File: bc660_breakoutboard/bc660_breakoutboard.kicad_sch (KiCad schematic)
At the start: 23 parts, among them J2 Conn_01x12_Pin, J3 Conn_Coaxial, J4 SIM8051-6-0-14-01-X-REVD, U1 BC660K-GL, U2 ESDS304DBVR

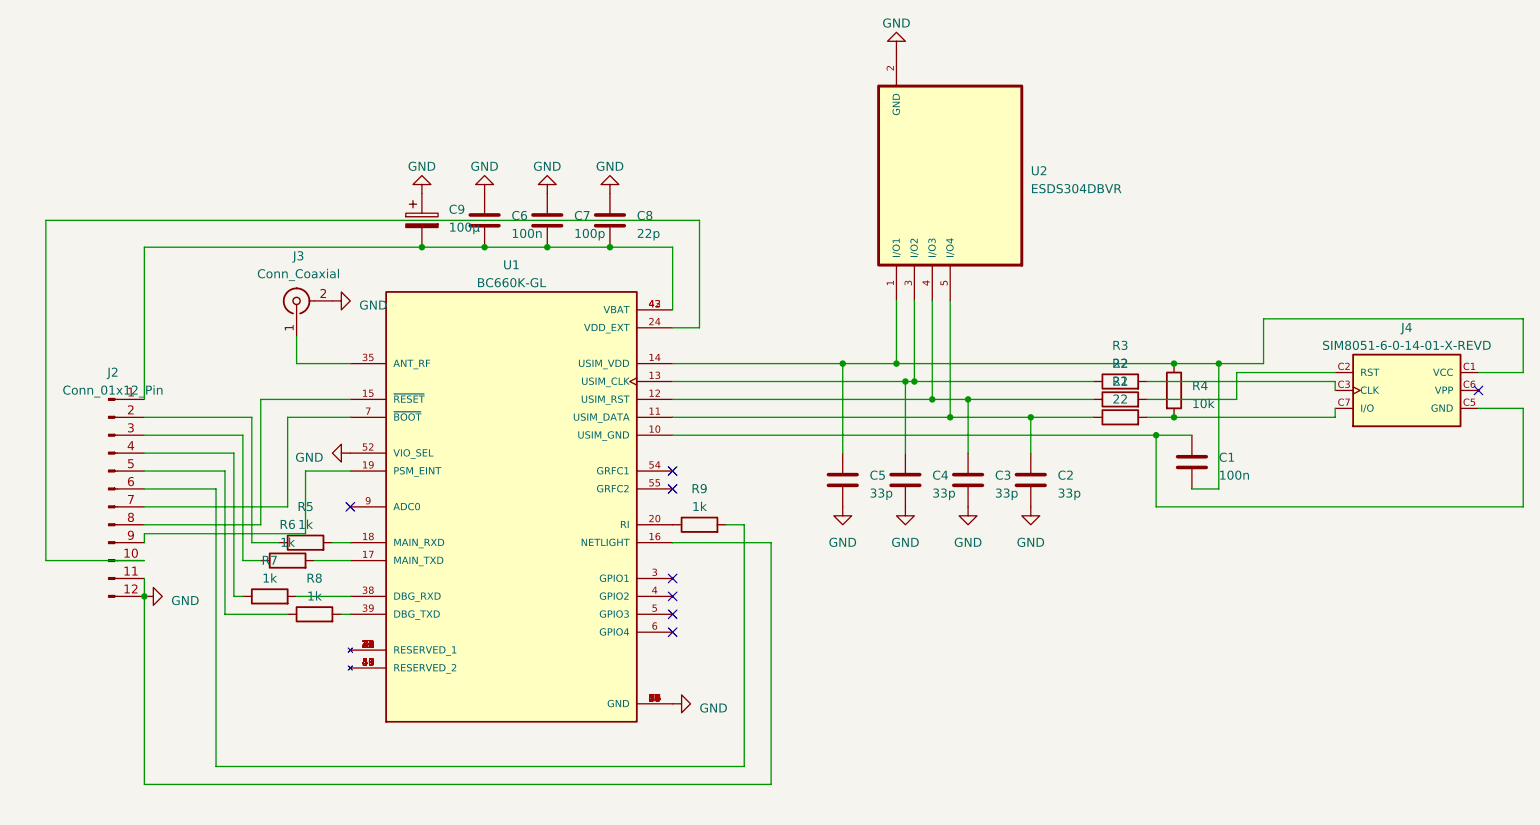
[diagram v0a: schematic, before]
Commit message: update pcb design
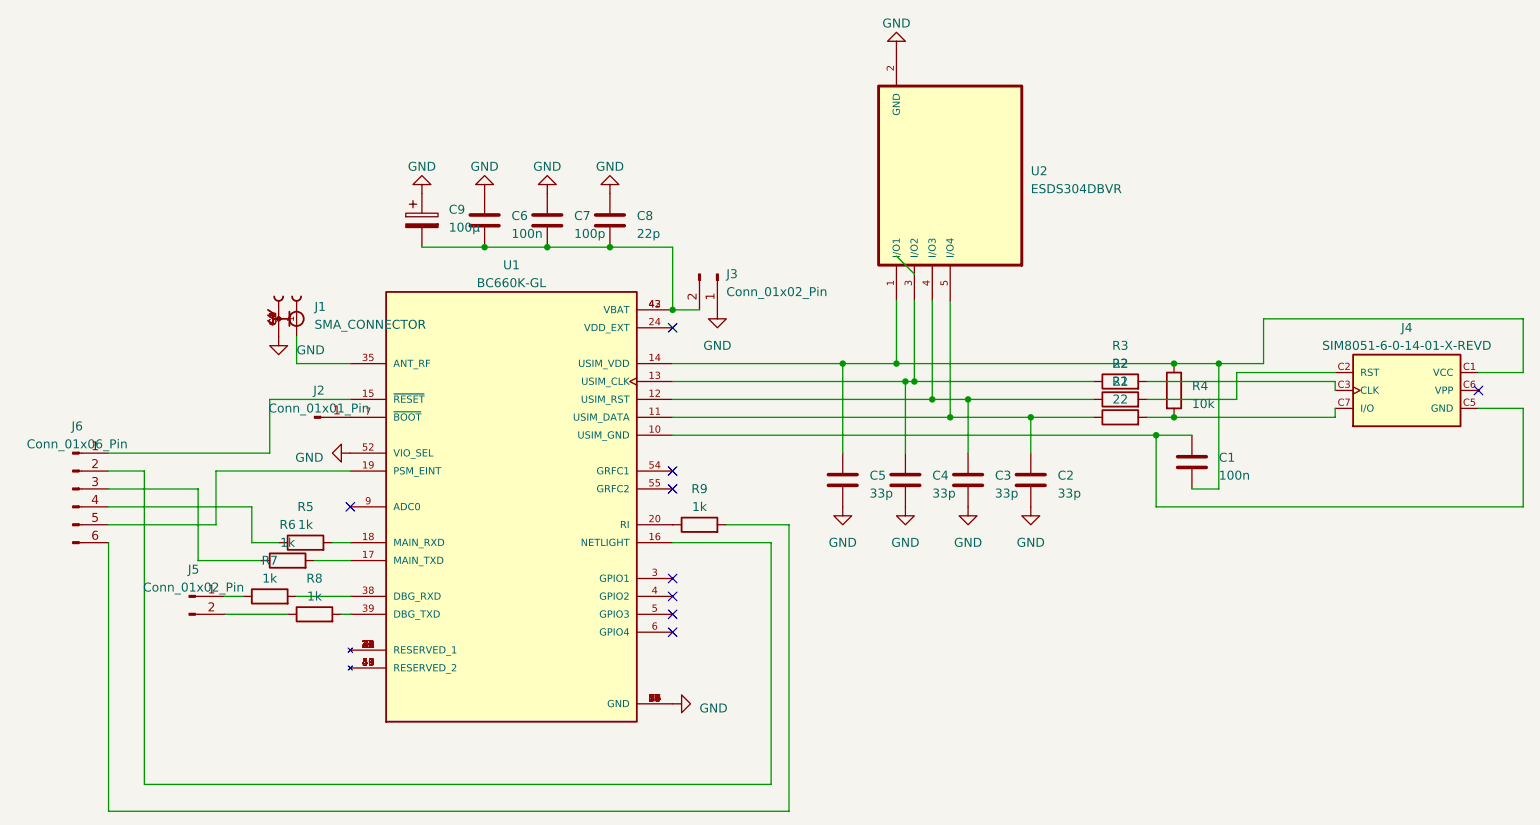
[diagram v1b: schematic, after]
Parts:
- removed J2: Conn_01x12_Pin, Connector_PinHeader_2.54mm:PinHeader_1x12_P2.54mm_Vertical, symbol Connector:Conn_01x12_Pin
- removed J3: Conn_Coaxial, symbol Connector:Conn_Coaxial
- added J1: SMA_CONNECTOR, SMA_CONNECTOR:LPRS_SMA_CONNECTOR, symbol SMA_CONNECTOR:SMA_CONNECTOR
- added J2: Conn_01x01_Pin, Connector_PinHeader_2.54mm:PinHeader_1x01_P2.54mm_Vertical, symbol Connector:Conn_01x01_Pin
- added J3, J5: Conn_01x02_Pin, Connector_PinHeader_2.54mm:PinHeader_1x02_P2.54mm_Vertical, symbol Connector:Conn_01x02_Pin
- added J6: Conn_01x06_Pin, Connector_PinHeader_2.54mm:PinHeader_1x06_P2.54mm_Vertical, symbol Connector:Conn_01x06_Pin
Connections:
- net GND: now also J1.G1, J1.G2, J1.G3, J1.G4, J3.1 (Pin_1); no longer U1.16 (NETLIGHT)
- net at R7.1: now also J5.1 (Pin_1)
- net at C6.2, C7.2, C8.2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: now also J3.2 (Pin_2)
- net at R5.1: now also J6.4 (Pin_4)
- net at R6.1: now also J6.3 (Pin_3)
- net at R8.1: now also J5.2 (Pin_2)
- net at R9.2: now also J6.6 (Pin_6)
- net at U1.7 (~{BOOT}): now also J2.1 (Pin_1)
- net at U1.15 (~{RESET}): now also J6.1 (Pin_1)
- net at U1.19 (PSM_EINT): now also J6.5 (Pin_5)
- net at U1.35 (ANT_RF): now also J1.1
- new net: J6.2 (Pin_2), U1.16 (NETLIGHT)
- no-connect marks 8 -> 9
